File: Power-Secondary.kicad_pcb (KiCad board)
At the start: 2 copper layers, 84 x 38 mm, 32 parts, among them J1 SUPP PWR, J2 DCDC SUPPLY, J3 FUSE +12V, Q1A1 SUP90P06-PCHANNEL-MOSFET, Q2B1 SUP90P06-PCHANNEL-MOSFET, U1 Opamp_Dual

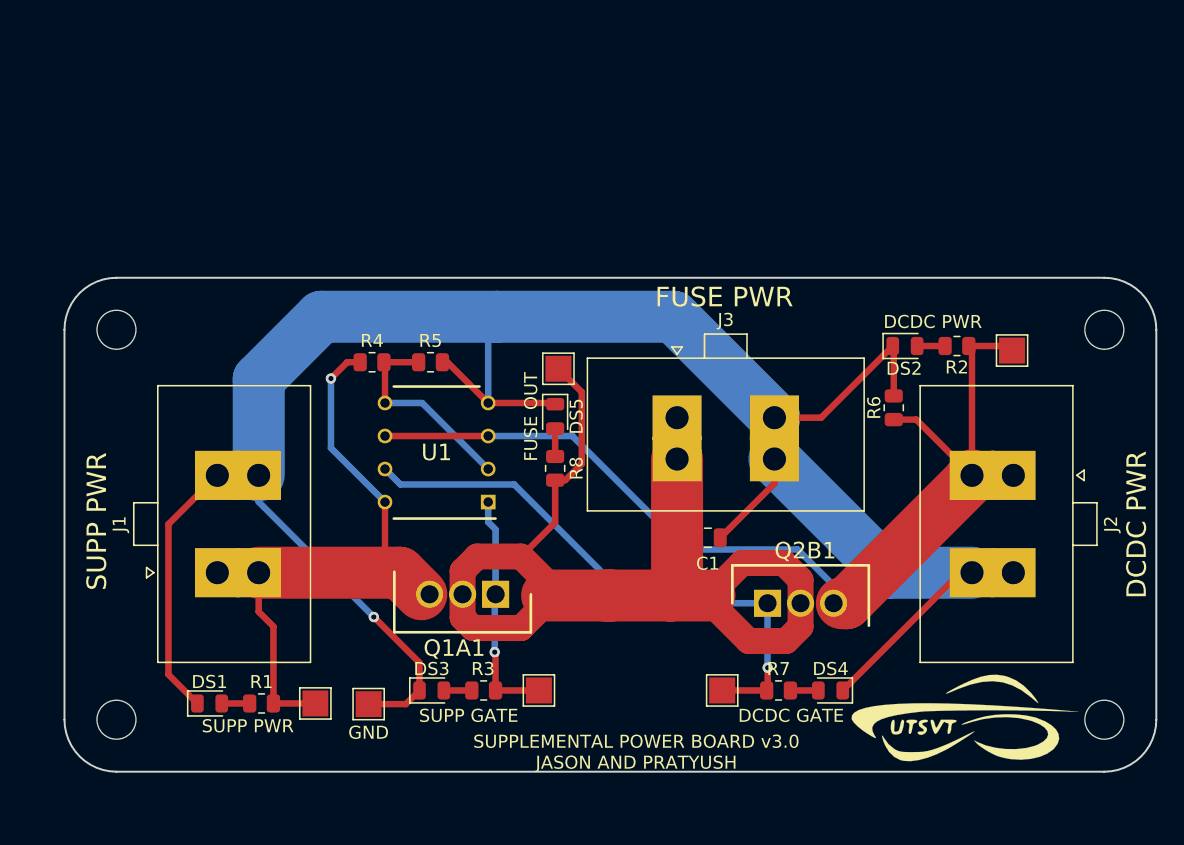
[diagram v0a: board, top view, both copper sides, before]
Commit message: v3 revision
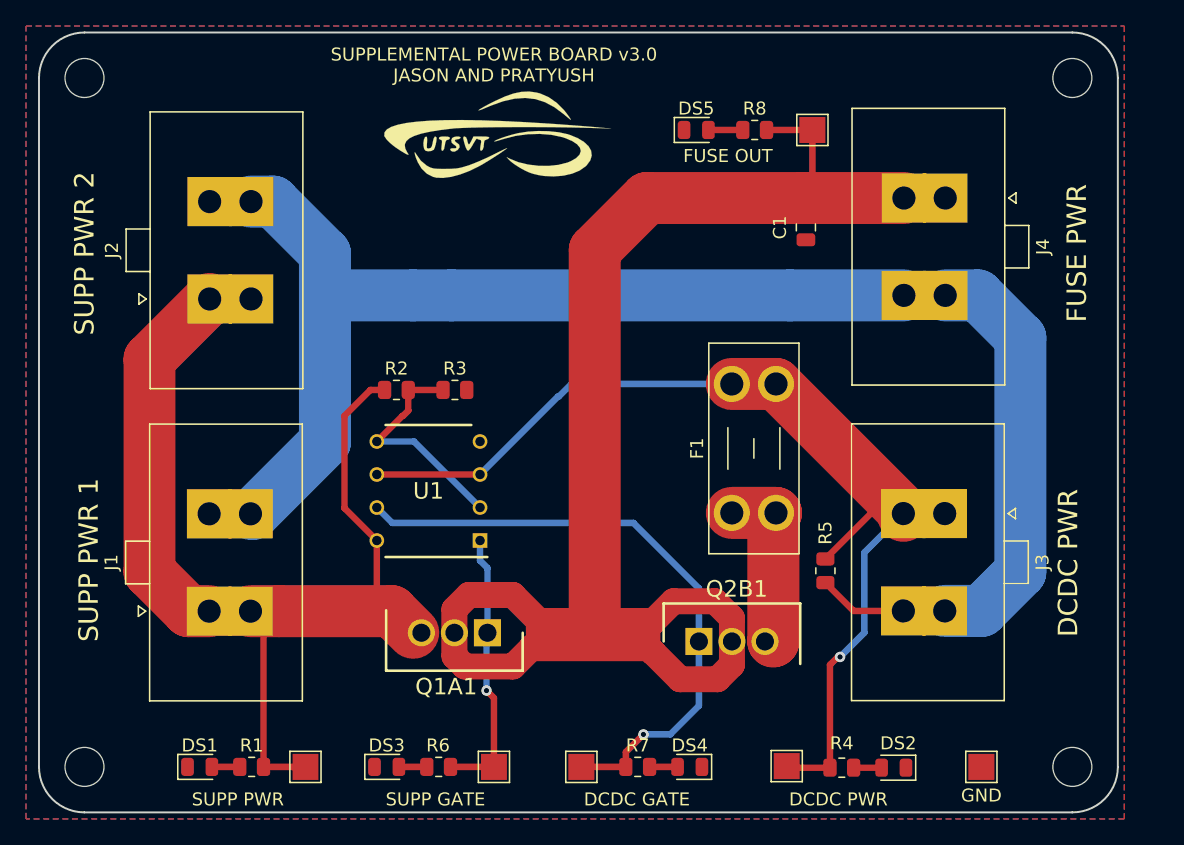
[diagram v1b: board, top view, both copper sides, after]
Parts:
- added F1: Fuse, Fuse:Fuseholder_Blade_Mini_Keystone_3568, F.Cu at (159.7, 104.4)
- added J2: SUPP PWR 2, Connector_Molex:Molex_Sabre_43160-0102_1x02_P7.49mm_Vertical, F.Cu at (122.7, 88.0)
- J1: value SUPP PWR -> SUPP PWR 1
- moved LOGO2 57.5 mm to (141.4, 75.5)
- moved LOGO1 48.5 mm to (132.9, 75.5)
- moved TP6 47.4 mm to (178.9, 124.0)
- moved TP2 36.4 mm to (163.9, 123.9), turned to 180 degrees
- moved R4 33.6 mm to (168.1, 124.0), turned to 0 degrees
- moved DS2 32.5 mm to (172.1, 124.0), turned to 180 degrees
- moved R8 30.2 mm to (161.4, 75.0), turned to 180 degrees
- moved TP5 26.8 mm to (165.9, 75.0)
- moved J4 26.6 mm to (172.9, 80.2), turned to -90 degrees
- moved C1 25.0 mm to (165.4, 82.5), turned to -90 degrees
- moved DS5 24.6 mm to (156.9, 75.0), turned to 0 degrees
- moved H1 19.5 mm to (109.9, 71.0)
- moved H2 19.5 mm to (185.9, 71.0)
- moved R5 13.6 mm to (166.9, 108.9), turned to -90 degrees
- moved DS4 12.3 mm to (156.4, 124.0)
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- renumbered J2 to J3, J3 to J4, R4 to R2, R5 to R3, R2 to R4, R6 to R5, R3 to R6
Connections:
- Q2B1 pad 3: DCDC_PWR -> Net-(F1-Pad1)
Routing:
- net GNDS: track 170.8 -> 120.2 mm, vias 1 -> 0
- net FUSE_OUT: track 83.9 -> 134.2 mm
- net SUPP_PWR: track 46.9 -> 78.1 mm, vias 1 -> 0
- net Net-(F1-Pad1): track 0.00 -> 14.1 mm
- net DCDC_PWR: track 76.2 -> 81.5 mm, vias 0 -> 1
- net DCDC_GATE: track 43.9 -> 48.2 mm
- net SUPP_GATE: track 18.1 -> 21.3 mm
- net V_REF: track 15.9 -> 17.8 mm
- net Net-(DS5-Pad2): track 2.15 -> 2.65 mm
- added copper zone on B.Cu, net GNDS
- added copper zone on F.Cu, net GNDS
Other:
- board size 84 x 38 mm -> 83 x 60 mm
- board text added: "SUPP PWR 1"
- board text added: "SUPP PWR 2"
